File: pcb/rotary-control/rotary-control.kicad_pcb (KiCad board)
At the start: 2 copper layers, 26 x 23.3 mm, 14 parts, among them J1 input, J2 output, J3 power, J4 neopixel, J5 AVR_SPI_PRG_6PTH, J6 encoder

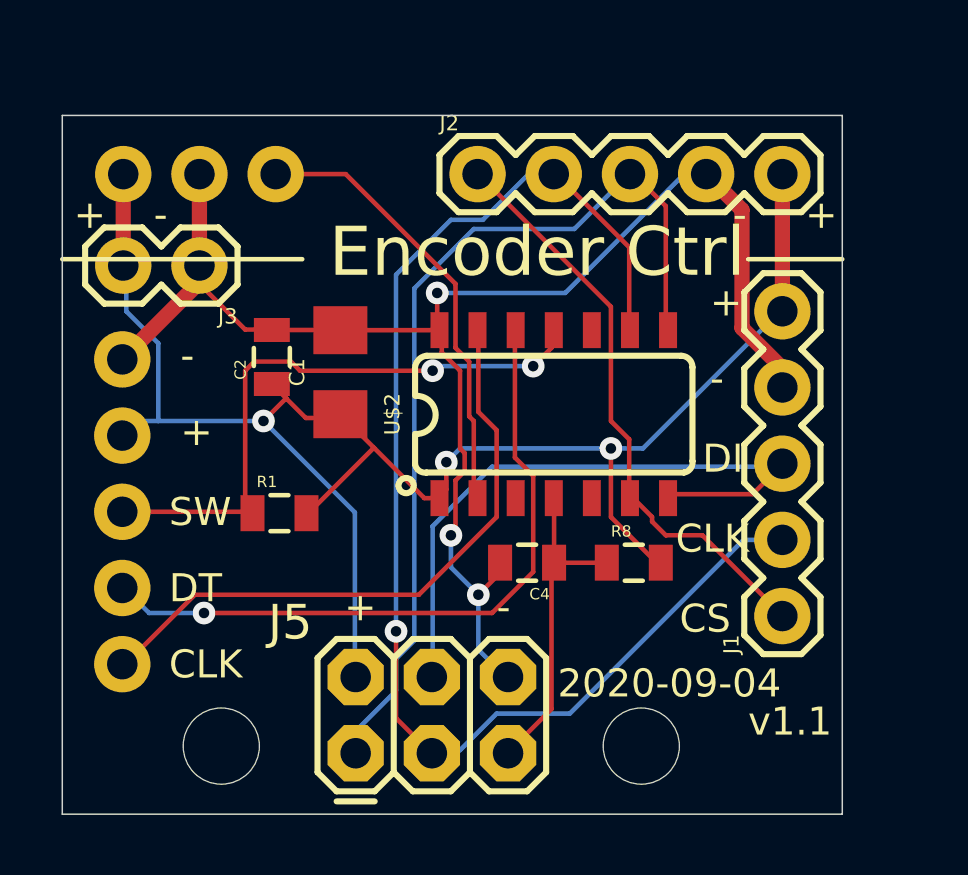
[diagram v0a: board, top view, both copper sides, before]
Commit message: Checkpoint PCB files.
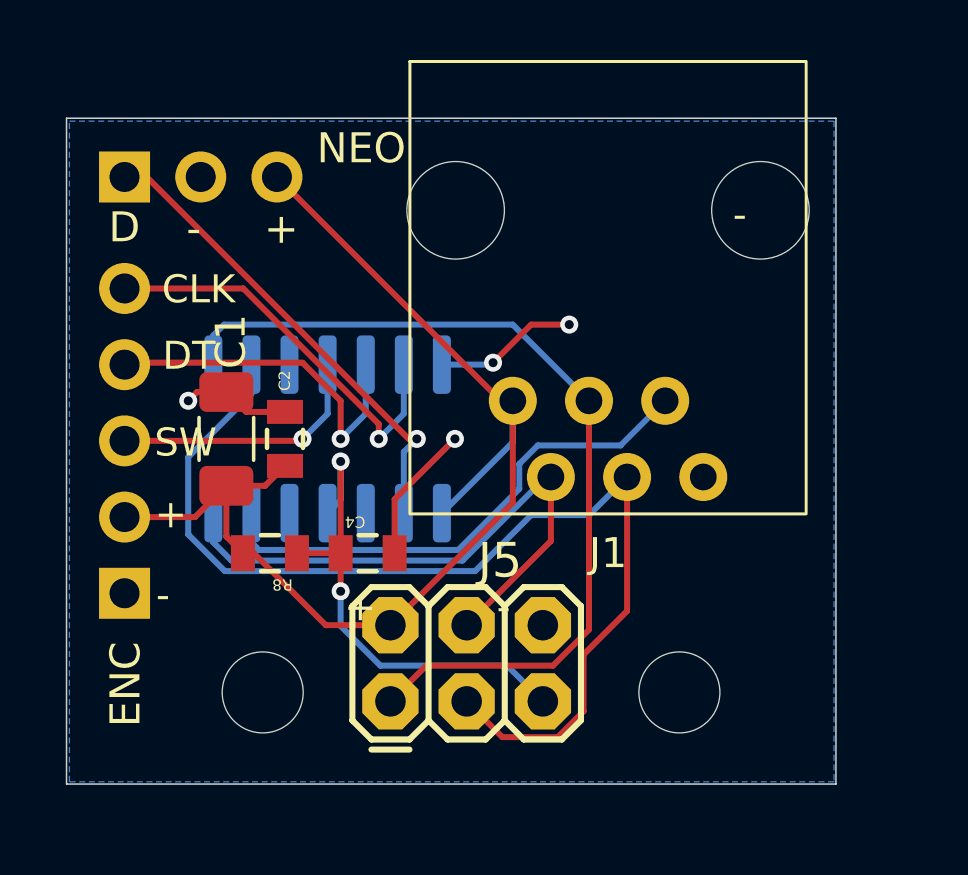
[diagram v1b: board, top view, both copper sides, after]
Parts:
- removed @HOLE0, @HOLE1: , 
- removed J2: output, rotary-control:1X05_513
- removed J3: power, rotary-control:1X02_513
- removed R1: 4K7, rotary-control:0805
- added H1: MountingHole, MountingHole:MountingHole_2.7mm_M2.5_Pad, F.Cu at (142.2, 112.6)
- added H2: MountingHole, MountingHole:MountingHole_2.7mm_M2.5_Pad, F.Cu at (156.1, 112.6)
- C1: value 10uF -> 10UF-1206-6.3V-20%; footprint rotary-control:1206_510 -> Capacitor_SMD:C_1206_3216Metric_Pad1.33x1.80mm_HandSolder
- J1: value input -> SPI-Comm; footprint rotary-control:1X05_513 -> Garth:RJ11-Straight
- J4: footprint rotary-control:1X03_513 -> Connector_PinHeader_2.54mm:PinHeader_1x03_P2.54mm_Vertical
- J6: footprint rotary-control:1X05_513 -> Connector_PinHeader_2.54mm:PinHeader_1x05_P2.54mm_Vertical
- U$2: footprint rotary-control:SO14_525 -> Package_SO:SOIC-14_3.9x8.7mm_P1.27mm; moved to B.Cu
- moved R8 12.1 mm to (142.4, 108.0), turned to 180 degrees
- moved J1 9.23 mm to (153.7, 102.9), turned to 0 degrees
- moved J6 7.80 mm to (137.6, 109.3), turned to 0 degrees
- moved U$2 6.95 mm to (144.3, 104.1), turned to 90 degrees
- moved C4 5.32 mm to (145.7, 108.0), turned to 0 degrees
- moved J4 5.04 mm to (137.6, 95.4), turned to -90 degrees
- moved C1 4.40 mm to (141.0, 104.1)
- moved C2 2.77 mm to (142.9, 104.1)
- moved J5 2.08 mm to (146.4, 112.9)
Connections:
- net ENC_CLK renamed /ENC_CLK
- net ENC_DT renamed /ENC_DT
- net ENC_SW renamed /ENC_SW
- net NEO_DIN renamed /NEO_DIN
- net RESET renamed /RESET
- J1 pad 1: CS -> VCC
- J1 pad 2: SCLK -> /DI
- J1 pad 3: DI -> /DO
- J1 pad 4: GND -> /SCLK
- J1 pad 5: VCC -> /CS
- J5 pad 1: DO -> /DO
- J5 pad 3: SCLK -> /SCLK
- J5 pad 4: DI -> /DI
- U$2 pad 10: (no net) -> unconnected-(U$2-(PCINT3/T0/ADC3)PA3-Pad10)
- U$2 pad 3: (no net) -> unconnected-(U$2-(PCINT9/XTAL2)PB1-Pad3)
- U$2 pad 5: (no net) -> unconnected-(U$2-(PCINT10/INT0/OC0A/CKOUT)PB2-Pad5)
- U$2 pad 6: CS -> /CS
- U$2 pad 7: DI -> /DI
- U$2 pad 8: DO -> /DO
- U$2 pad 9: SCLK -> /SCLK
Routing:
- net SCLK: track 44.1 -> 0.00 mm, vias 1 -> 0
- net GND: track 50.9 -> 13.8 mm, vias 3 -> 4
- net /SCLK: track 0.00 -> 36.1 mm
- net DO: track 30.9 -> 0.00 mm
- net /DO: track 0.00 -> 29.9 mm
- net DI: track 21.9 -> 0.00 mm
- net /DI: track 0.00 -> 19.7 mm
- net CS: track 19.7 -> 0.00 mm
- net VCC: track 58.8 -> 39.3 mm, vias 3 -> 0
- net /CS: track 0.00 -> 17.4 mm
- net /ENC_SW: track 20.7 -> 8.78 mm, vias 2 -> 1
- net /ENC_DT: track 22.9 -> 11.8 mm
- net /ENC_CLK: track 21.0 -> 13.7 mm, vias 0 -> 1
- net /RESET: track 10.9 -> 16.6 mm, vias 0 -> 2
- net /NEO_DIN: track 15.0 -> 16.0 mm, vias 0 -> 1
- added copper zone on B.Cu, net GND
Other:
- board size 26 x 23.3 mm -> 25.6 x 22.2 mm
- board text added: "2024-06-13"
- board text added: "D"
- board text added: "ENC"
- board text added: "NEO"
- board text added: "v2.0"
- board text removed: "2020-09-04"
- board text removed: "CS"
- board text removed: "DI"
- board text removed: "v1.1"
